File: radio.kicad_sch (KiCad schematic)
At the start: 35 parts, among them Q1 BSS138W-7-F, U3 SX1276, X1 AS183-92LF, Y1 ECS-TXO-25CSMV-320-AM-TR

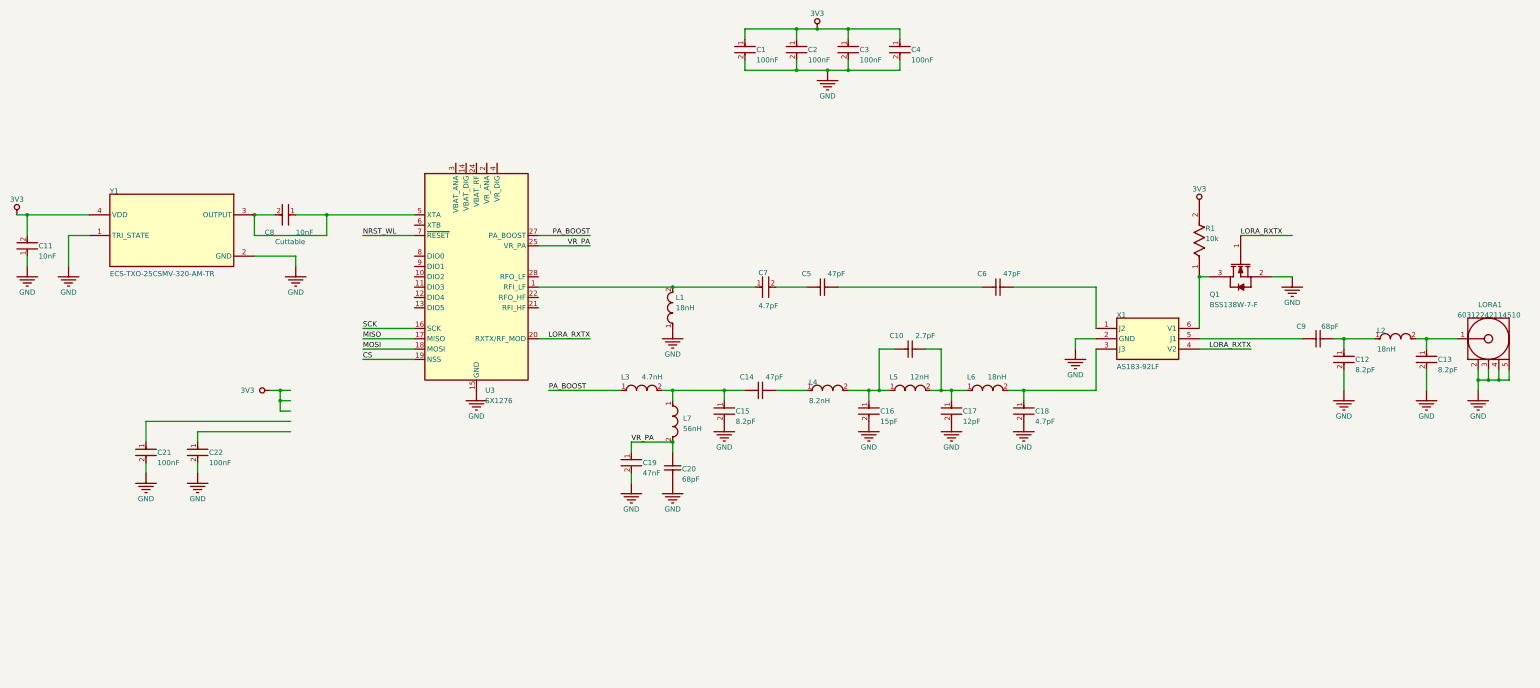
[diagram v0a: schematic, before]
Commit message: proper formating
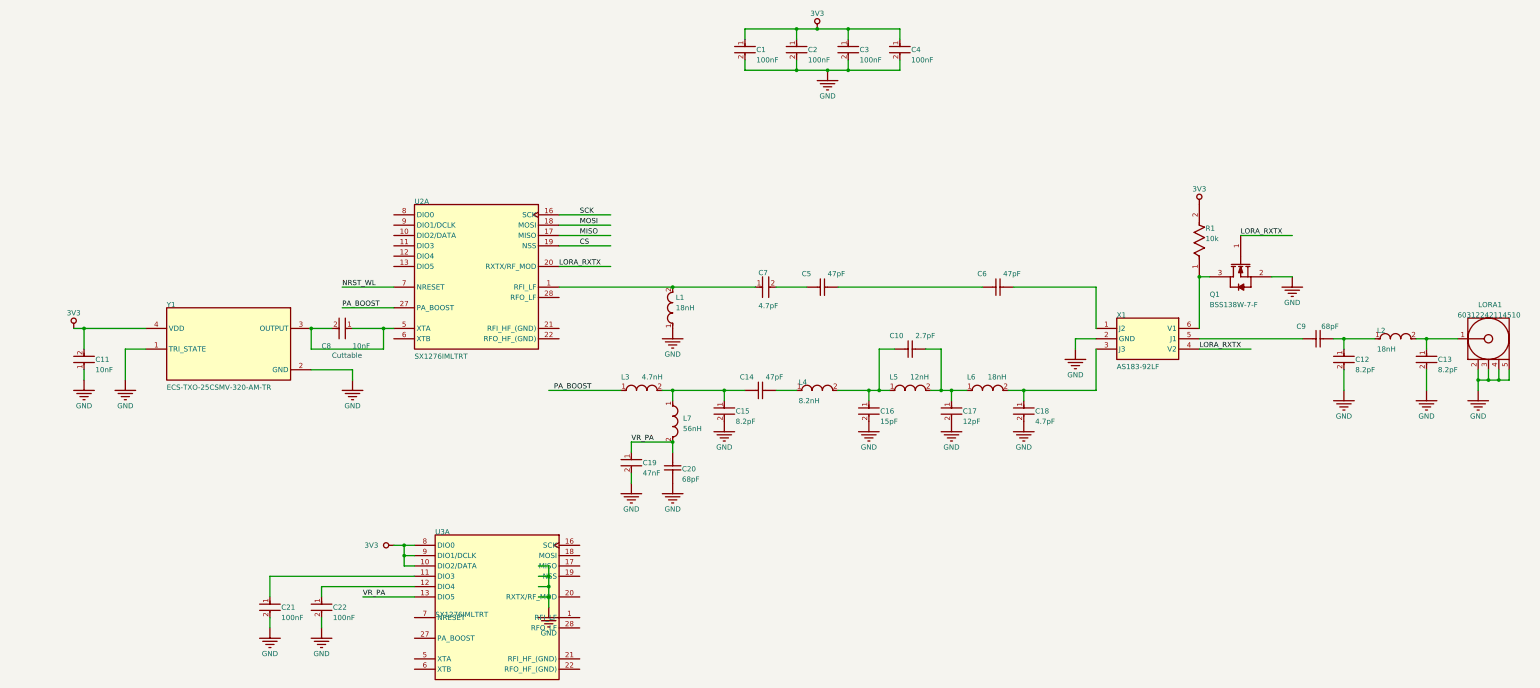
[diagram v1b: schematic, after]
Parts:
- removed U3: SX1276, Package_DFN_QFN:QFN-28-1EP_6x6mm_P0.65mm_EP4.8x4.8mm, symbol RF:SX1276
- added U2, U3: SX1276IMLTRT, SMTC-QFN-28_V, symbol Altium Content Vault:root_0_SMTC-SX127X-QFN-28_Altium Content Vault
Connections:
- net 3V3: now also U3.10 (DIO2/DATA), U3.8 (DIO0), U3.9 (DIO1/DCLK)
- net CS: now also U2.19 (NSS)
- net LORA_RXTX: now also U2.20 (RXTX/RF_MOD)
- net MISO: now also U2.17 (MISO)
- net MOSI: now also U2.18 (MOSI)
- net NRST_WL: now also U2.7 (NRESET)
- net PA_BOOST: now also U2.27 (PA_BOOST)
- net SCK: now also U2.16 (SCK)
- net VR_PA: now also U3.13 (DIO5)
- net at C7.1, L1.2: now also U2.1 (RFI_LF)
- net at C8.1, C8.2, Y1.3 (OUTPUT): now also U2.5 (XTA)
- net at C21.1: now also U3.11 (DIO3)
- net at C22.1: now also U3.12 (DIO4)
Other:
- moved on the sheet: C11, C21, C22, C8, L4, Y1
